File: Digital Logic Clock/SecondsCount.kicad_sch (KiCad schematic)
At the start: 19 parts, among them U1 4081

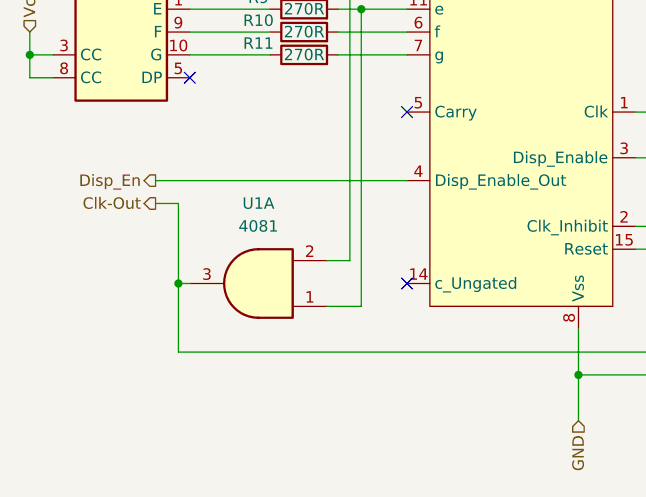
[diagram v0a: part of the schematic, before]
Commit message: Clock Project
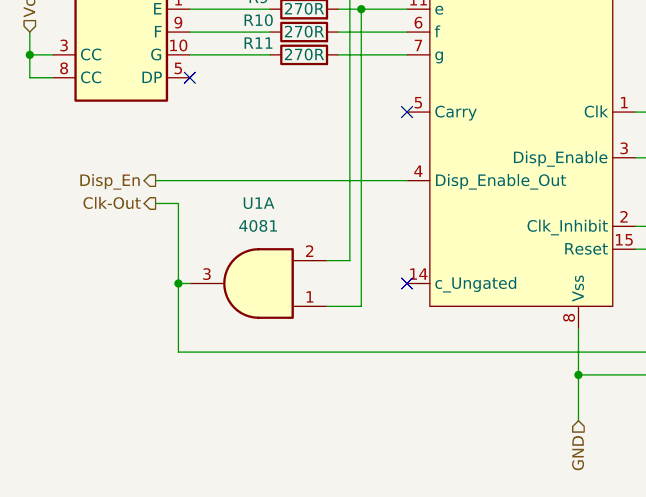
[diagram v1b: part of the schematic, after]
